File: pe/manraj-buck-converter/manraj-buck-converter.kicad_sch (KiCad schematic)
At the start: 10 parts, among them U1 AP62300WU-7

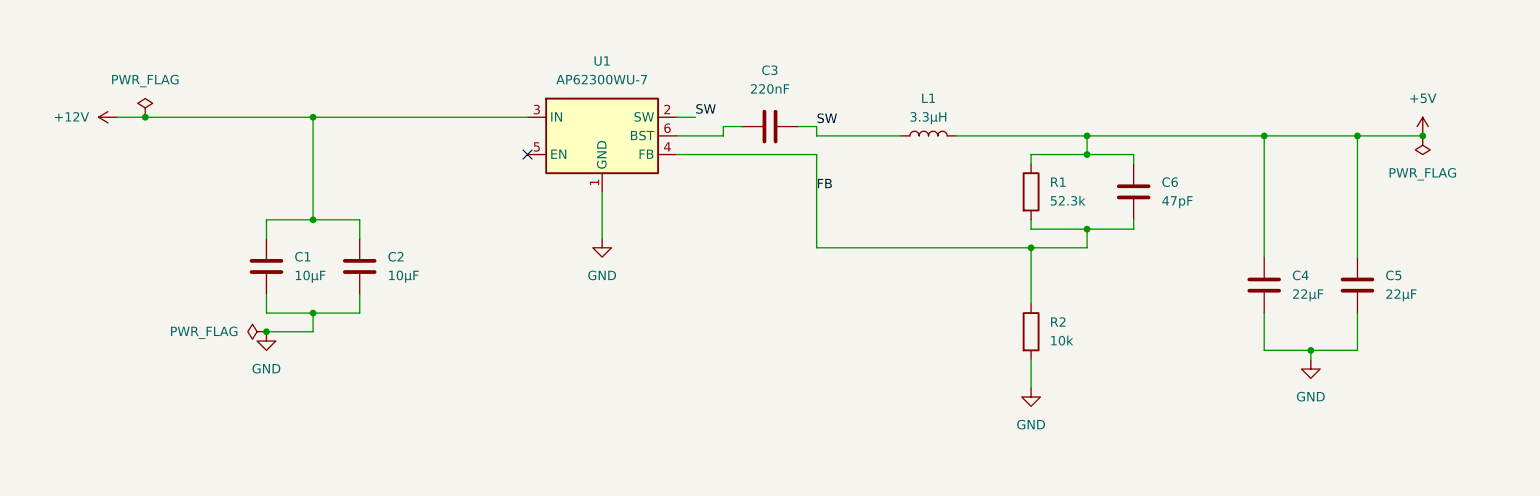
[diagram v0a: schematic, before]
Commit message: PCB finished
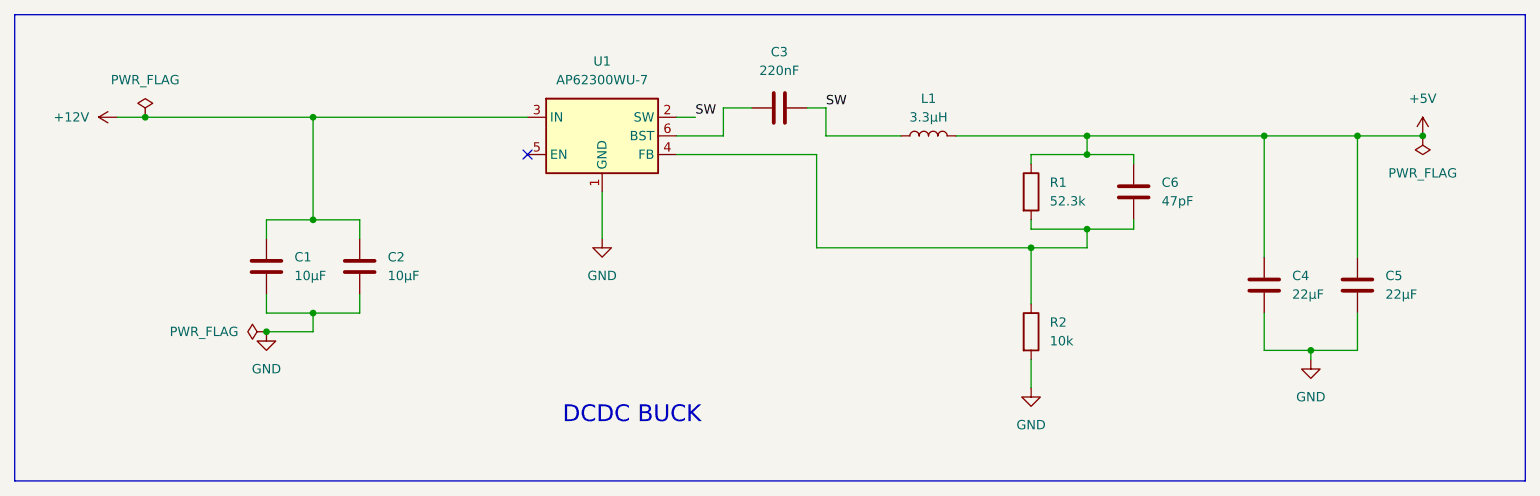
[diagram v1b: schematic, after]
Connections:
- net FB: no longer names the net of C6.2, R1.2, R2.1, U1.4 (FB)
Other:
- note added: "DCDC BUCK"
- moved on the sheet: C3
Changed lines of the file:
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@@
 		(comment 3 "${COMMENT2}")
+	)
+	(rectangle
+		(start 52.07 60.96)
+		(end 257.81 124.46)
+		(stroke
+			(width 0)
+			(type default)
+		)
+		(fill
+			(type none)
+		)
+	)
+	(text "DCDC BUCK\n\n"
+		(exclude_from_sim no)
+		(at 136.144 117.348 0)
+		(effects
+			(font
+				(size 2.286 2.286)
+			)
+		)
 	)
 	(junction
@@
 	(wire
 		(pts
+			(xy 162.56 77.47) (xy 172.72 77.47)
+		)
+		(stroke
+			(width 0)
+			(type default)
+		)
+	)
+	(wire
+		(pts
 			(xy 92.71 101.6) (xy 99.06 101.6)
 		)
@@
 	(wire
 		(pts
-			(xy 161.29 77.47) (xy 161.29 76.2)
+			(xy 162.56 73.66) (xy 162.56 77.47)
 		)
 		(stroke
@@
 	(wire
 		(pts
-			(xy 158.75 76.2) (xy 161.29 76.2)
+			(xy 160.02 73.66) (xy 162.56 73.66)
 		)
 		(stroke
@@
 	(wire
 		(pts
-			(xy 172.72 77.47) (xy 161.29 77.47)
-		)
-		(stroke
-			(width 0)
-			(type default)
-		)
-	)
-	(wire
-		(pts
 			(xy 234.95 101.6) (xy 234.95 106.68)
 		)
@@
 	(wire
 		(pts
-			(xy 148.59 77.47) (xy 148.59 76.2)
+			(xy 148.59 77.47) (xy 148.59 73.66)
 		)
 		(stroke
@@
 	(wire
 		(pts
-			(xy 148.59 76.2) (xy 151.13 76.2)
+			(xy 148.59 73.66) (xy 152.4 73.66)
 		)
 		(stroke
@@
 		)
 	)
-	(label "FB"
-		(at 161.29 85.09 0)
-		(effects
-			(font
-				(size 1.27 1.27)
-			)
-			(justify left bottom)
-		)
-	)
 	(label "SW"
-		(at 161.29 76.2 0)
+		(at 162.56 73.66 0)
 		(effects
 			(font
@@
 	(symbol
 		(lib_id "Device:C")
-		(at 154.94 76.2 90)
+		(at 156.21 73.66 90)
 		(unit 1)
 		(body_style 1)
@@
 		(fields_autoplaced yes)
 		(property "Reference" "C3"
-			(at 154.94 68.58 90)
+			(at 156.21 66.04 90)
 			(show_name no)
 			(do_not_autoplace no)
@@
 		)
 		(property "Value" "220nF"
-			(at 154.94 71.12 90)
+			(at 156.21 68.58 90)
 			(show_name no)
 			(do_not_autoplace no)
@@
 		)
 		(property "Footprint" "Capacitor_SMD:C_0603_1608Metric_Pad1.08x0.95mm_HandSolder"
-			(at 158.75 75.2348 0)
+			(at 160.02 72.6948 0)
 			(hide yes)
 			(show_name no)
@@
 		)
 		(property "Datasheet" "https://pim.murata.com/asset/pim4/ceramicCapacitorSMD/GCM188R71H224KA64-01A-EN_PDF_CERAMICCAPACITORSMD"
-			(at 154.94 76.2 0)
+			(at 156.21 73.66 0)
 			(hide yes)
 			(show_name no)
@@
 		)
 		(property "Description" "Unpolarized capacitor, 220nF, 50v, X7R, 10%, 0603, AEC-Q200"
-			(at 154.94 76.2 0)
+			(at 156.21 73.66 0)
 			(hide yes)
 			(show_name no)
@@
 		)
 		(property "Digikey Part Number" "490-13307-1-ND"
-			(at 154.94 76.2 0)
+			(at 156.21 73.66 0)
 			(hide yes)
 			(show_name no)
@@
 		)
 		(property "Digikey URL" "https://www.digikey.com/en/products/detail/murata-electronics/gcm188r71h224ka64j/4903960"
-			(at 154.94 76.2 0)
+			(at 156.21 73.66 0)
 			(hide yes)
 			(show_name no)
@@
 		)
 		(property "Manufacturer" "Murata Electronics"
-			(at 154.94 76.2 0)
+			(at 156.21 73.66 0)
 			(hide yes)
 			(show_name no)
@@
 		)
 		(property "Manufacturer Part Number" "GCM188R71H224KA64J"
-			(at 154.94 76.2 0)
-			(hide yes)
-			(show_name no)
+			(at 156.21 73.66 0)
+			(hide yes)
+			(show_name no)
